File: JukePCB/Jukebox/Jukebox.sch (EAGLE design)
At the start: 33 parts, among them J1 RJ45

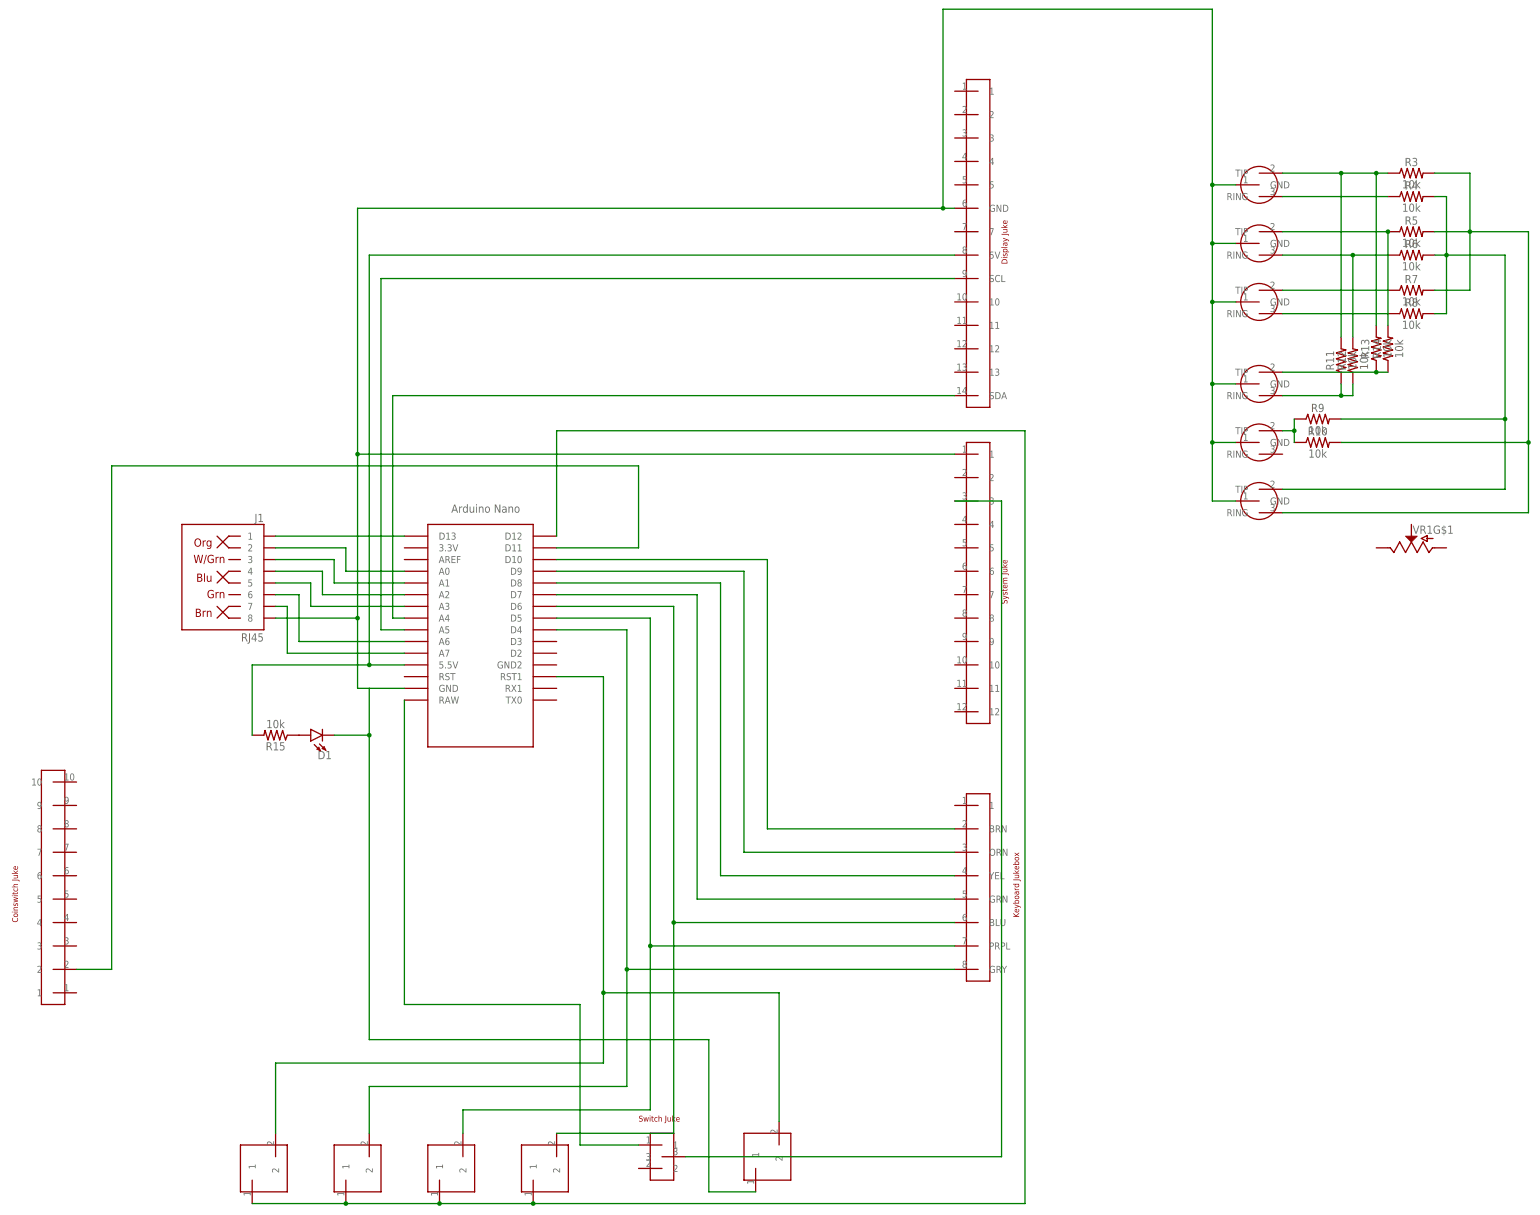
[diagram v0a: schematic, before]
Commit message: PCB UPDATE 2
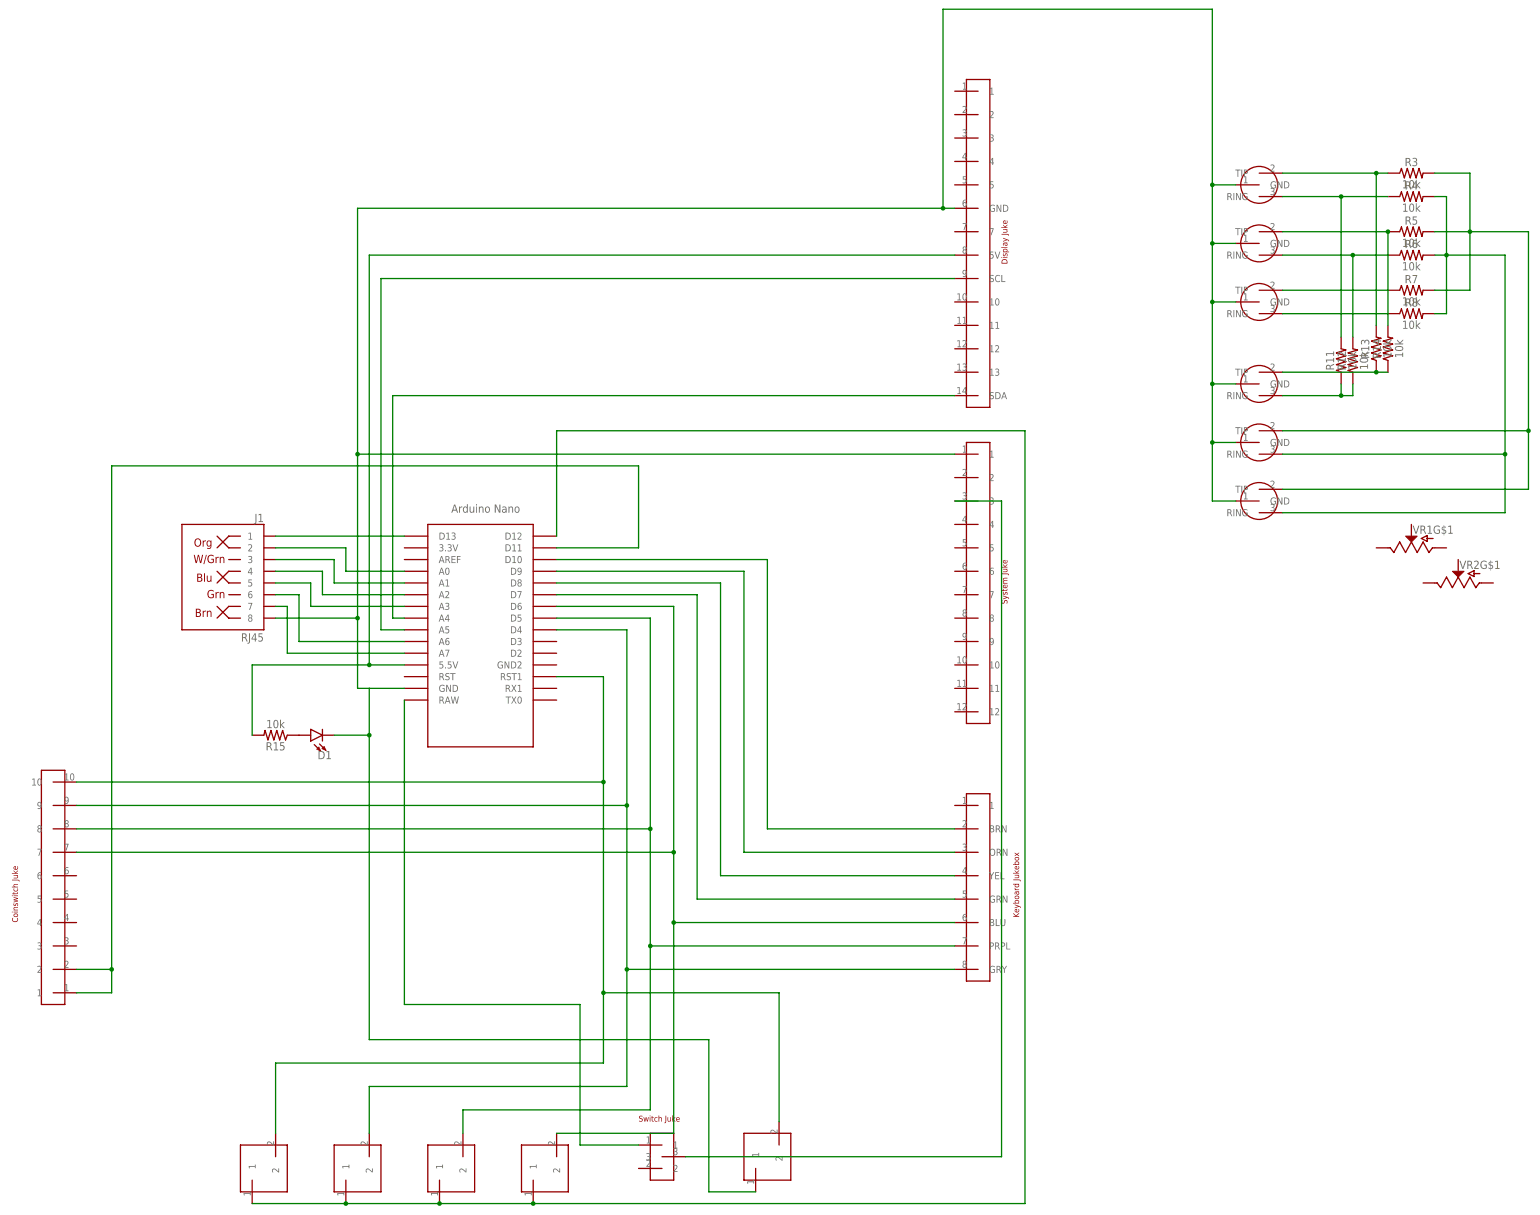
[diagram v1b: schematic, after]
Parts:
- removed R10, R9: 10k, SparkFun-Resistors:10KOHM-HORIZ-1/4W-1%
- added VR2: (no value), SparkFun-Resistors:POTENTIOMETER_DUAL-PTH-12MM-1/20W-20%
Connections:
- removed net N$22: R10.1, R9.1, U$16.TIP
- net N$1: now also U$5.9
- net N$11: now also U$5.1
- net N$14: no longer R11.2
- net N$15: now also R11.2
- net N$2: now also U$5.8
- net N$23: now also U$16.RING, U$2.RING; no longer R9.2, U$2.TIP
- net N$24: now also U$16.TIP, U$2.TIP; no longer R10.2, U$2.RING
- net N$3: now also U$5.7
- net N$9: now also U$5.10
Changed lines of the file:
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@@
 <part name="R8" library="SparkFun-Resistors" deviceset="10KOHM" device="-HORIZ-1/4W-1%" value="10k"/>
 <part name="VR1" library="SparkFun-Resistors" deviceset="POTENTIOMETER_DUAL" device="-PTH-12MM-1/20W-20%"/>
-<part name="R9" library="SparkFun-Resistors" deviceset="10KOHM" device="-HORIZ-1/4W-1%" value="10k"/>
-<part name="R10" library="SparkFun-Resistors" deviceset="10KOHM" device="-HORIZ-1/4W-1%" value="10k"/>
 <part name="U$2" library="Jukebox" deviceset="JUKEHEADPHONE" device=""/>
 <part name="R11" library="SparkFun-Resistors" deviceset="10KOHM" device="-HORIZ-1/4W-1%" value="10k"/>
@@
 <part name="R15" library="SparkFun-Resistors" deviceset="10KOHM" device="-HORIZ-1/4W-1%" value="10k"/>
 <part name="D1" library="SparkFun-LED" deviceset="LED" device="5MM"/>
+<part name="VR2" library="SparkFun-Resistors" deviceset="POTENTIOMETER_DUAL" device="-PTH-12MM-1/20W-20%"/>
 </parts>
 <sheets>
@@
 <instance part="R8" gate="G$1" x="226.06" y="55.88"/>
 <instance part="VR1" gate="G$1" x="226.06" y="5.08" rot="R90"/>
-<instance part="R9" gate="G$1" x="205.74" y="33.02"/>
-<instance part="R10" gate="G$1" x="205.74" y="27.94"/>
 <instance part="U$2" gate="G$1" x="193.04" y="15.24" rot="R90"/>
 <instance part="R11" gate="G$1" x="210.82" y="45.72" rot="R90"/>
@@
 <instance part="R15" gate="G$1" x="-20.32" y="-35.56" rot="R180"/>
 <instance part="D1" gate="G$1" x="-12.7" y="-35.56" rot="R90"/>
+<instance part="VR2" gate="G$1" x="236.22" y="-2.54" rot="R90"/>
 </instances>
 <busses>
@@
 <pinref part="U$6" gate="G$1" pin="GRY"/>
 <wire x1="127" y1="-86.36" x2="55.88" y2="-86.36" width="0.1524" layer="91"/>
-<wire x1="55.88" y1="-86.36" x2="55.88" y2="-12.7" width="0.1524" layer="91"/>
+<wire x1="55.88" y1="-86.36" x2="55.88" y2="-50.8" width="0.1524" layer="91"/>
 <pinref part="U$1" gate="G$1" pin="D4"/>
+<wire x1="55.88" y1="-50.8" x2="55.88" y2="-12.7" width="0.1524" layer="91"/>
 <wire x1="55.88" y1="-12.7" x2="40.64" y2="-12.7" width="0.1524" layer="91"/>
 <pinref part="U$10" gate="G$1" pin="2"/>
@@
 <wire x1="55.88" y1="-111.76" x2="55.88" y2="-86.36" width="0.1524" layer="91"/>
 <junction x="55.88" y="-86.36"/>
+<pinref part="U$5" gate="G$1" pin="9"/>
+<wire x1="-63.5" y1="-50.8" x2="55.88" y2="-50.8" width="0.1524" layer="91"/>
+<junction x="55.88" y="-50.8"/>
 </segment>
 </net>
@@
 <pinref part="U$6" gate="G$1" pin="PRPL"/>
 <wire x1="127" y1="-81.28" x2="60.96" y2="-81.28" width="0.1524" layer="91"/>
-<wire x1="60.96" y1="-81.28" x2="60.96" y2="-10.16" width="0.1524" layer="91"/>
+<wire x1="60.96" y1="-81.28" x2="60.96" y2="-55.88" width="0.1524" layer="91"/>
 <pinref part="U$1" gate="G$1" pin="D5"/>
+<wire x1="60.96" y1="-55.88" x2="60.96" y2="-10.16" width="0.1524" layer="91"/>
 <wire x1="60.96" y1="-10.16" x2="40.64" y2="-10.16" width="0.1524" layer="91"/>
 <pinref part="U$11" gate="G$1" pin="2"/>
@@
 <wire x1="60.96" y1="-116.84" x2="60.96" y2="-81.28" width="0.1524" layer="91"/>
 <junction x="60.96" y="-81.28"/>
+<pinref part="U$5" gate="G$1" pin="8"/>
+<wire x1="-63.5" y1="-55.88" x2="60.96" y2="-55.88" width="0.1524" layer="91"/>
+<junction x="60.96" y="-55.88"/>
 </segment>
 </net>
@@
 <pinref part="U$6" gate="G$1" pin="BLU"/>
 <wire x1="127" y1="-76.2" x2="66.04" y2="-76.2" width="0.1524" layer="91"/>
-<wire x1="66.04" y1="-76.2" x2="66.04" y2="-7.62" width="0.1524" layer="91"/>
+<wire x1="66.04" y1="-76.2" x2="66.04" y2="-60.96" width="0.1524" layer="91"/>
 <pinref part="U$1" gate="G$1" pin="D6"/>
+<wire x1="66.04" y1="-60.96" x2="66.04" y2="-7.62" width="0.1524" layer="91"/>
 <wire x1="66.04" y1="-7.62" x2="40.64" y2="-7.62" width="0.1524" layer="91"/>
 <pinref part="U$12" gate="G$1" pin="2"/>
@@
 <wire x1="66.04" y1="-121.92" x2="66.04" y2="-76.2" width="0.1524" layer="91"/>
 <junction x="66.04" y="-76.2"/>
+<pinref part="U$5" gate="G$1" pin="7"/>
+<wire x1="-63.5" y1="-60.96" x2="66.04" y2="-60.96" width="0.1524" layer="91"/>
+<junction x="66.04" y="-60.96"/>
 </segment>
 </net>
@@
 <wire x1="88.9" y1="-119.38" x2="88.9" y2="-91.44" width="0.1524" layer="91"/>
 <wire x1="88.9" y1="-91.44" x2="50.8" y2="-91.44" width="0.1524" layer="91"/>
-<wire x1="50.8" y1="-91.44" x2="50.8" y2="-22.86" width="0.1524" layer="91"/>
+<wire x1="50.8" y1="-91.44" x2="50.8" y2="-45.72" width="0.1524" layer="91"/>
 <pinref part="U$1" gate="G$1" pin="RST1"/>
+<wire x1="50.8" y1="-45.72" x2="50.8" y2="-22.86" width="0.1524" layer="91"/>
 <wire x1="50.8" y1="-22.86" x2="40.64" y2="-22.86" width="0.1524" layer="91"/>
 <pinref part="U$9" gate="G$1" pin="2"/>
@@
 <wire x1="50.8" y1="-106.68" x2="50.8" y2="-91.44" width="0.1524" layer="91"/>
 <junction x="50.8" y="-91.44"/>
+<pinref part="U$5" gate="G$1" pin="10"/>
+<wire x1="-63.5" y1="-45.72" x2="50.8" y2="-45.72" width="0.1524" layer="91"/>
+<junction x="50.8" y="-45.72"/>
 </segment>
 </net>
@@
 <pinref part="U$5" gate="G$1" pin="2"/>
 <wire x1="-55.88" y1="-86.36" x2="-63.5" y2="-86.36" width="0.1524" layer="91"/>
+<pinref part="U$5" gate="G$1" pin="1"/>
+<wire x1="-63.5" y1="-91.44" x2="-55.88" y2="-91.44" width="0.1524" layer="91"/>
+<wire x1="-55.88" y1="-91.44" x2="-55.88" y2="-86.36" width="0.1524" layer="91"/>
+<junction x="-55.88" y="-86.36"/>
 </segment>
 </net>
@@
 <segment>
 <pinref part="AUXIN" gate="G$1" pin="TIP"/>
-<wire x1="198.12" y1="86.36" x2="210.82" y2="86.36" width="0.1524" layer="91"/>
+<wire x1="198.12" y1="86.36" x2="218.44" y2="86.36" width="0.1524" layer="91"/>
 <pinref part="R3" gate="G$1" pin="1"/>
-<wire x1="210.82" y1="86.36" x2="218.44" y2="86.36" width="0.1524" layer="91"/>
 <wire x1="218.44" y1="86.36" x2="220.98" y2="86.36" width="0.1524" layer="91"/>
 <wire x1="218.44" y1="86.36" x2="218.44" y2="53.34" width="0.1524" layer="91"/>
 <junction x="218.44" y="86.36"/>
 <pinref part="R13" gate="G$1" pin="2"/>
+</segment>
+</net>
+<net name="N$15" class="0">
+<segment>
+<pinref part="AUXIN" gate="G$1" pin="RING"/>
+<wire x1="198.12" y1="81.28" x2="210.82" y2="81.28" width="0.1524" layer="91"/>
+<pinref part="R4" gate="G$1" pin="1"/>
 <pinref part="R11" gate="G$1" pin="2"/>
-<wire x1="210.82" y1="50.8" x2="210.82" y2="86.36" width="0.1524" layer="91"/>
-<junction x="210.82" y="86.36"/>
-</segment>
-</net>
-<net name="N$15" class="0">
-<segment>
-<pinref part="AUXIN" gate="G$1" pin="RING"/>
-<wire x1="198.12" y1="81.28" x2="220.98" y2="81.28" width="0.1524" layer="91"/>
-<pinref part="R4" gate="G$1" pin="1"/>
+<wire x1="210.82" y1="81.28" x2="220.98" y2="81.28" width="0.1524" layer="91"/>
+<wire x1="210.82" y1="50.8" x2="210.82" y2="81.28" width="0.1524" layer="91"/>
+<junction x="210.82" y="81.28"/>
 </segment>
 </net>
@@
 </segment>
 </net>
-<net name="N$22" class="0">
-<segment>
-<pinref part="U$16" gate="G$1" pin="TIP"/>
-<wire x1="198.12" y1="30.48" x2="200.66" y2="30.48" width="0.1524" layer="91"/>
-<pinref part="R9" gate="G$1" pin="1"/>
-<wire x1="200.66" y1="30.48" x2="200.66" y2="33.02" width="0.1524" layer="91"/>
-<pinref part="R10" gate="G$1" pin="1"/>
-<wire x1="200.66" y1="30.48" x2="200.66" y2="27.94" width="0.1524" layer="91"/>
-<junction x="200.66" y="30.48"/>
-</segment>
-</net>
 <net name="N$23" class="0">
 <segment>
-<pinref part="R9" gate="G$1" pin="2"/>
 <pinref part="R8" gate="G$1" pin="2"/>
 <wire x1="231.14" y1="55.88" x2="233.68" y2="55.88" width="0.1524" layer="91"/>
@@
 <wire x1="233.68" y1="81.28" x2="231.14" y2="81.28" width="0.1524" layer="91"/>
 <wire x1="233.68" y1="68.58" x2="246.38" y2="68.58" width="0.1524" layer="91"/>
-<wire x1="246.38" y1="68.58" x2="246.38" y2="33.02" width="0.1524" layer="91"/>
-<pinref part="U$2" gate="G$1" pin="TIP"/>
-<wire x1="246.38" y1="33.02" x2="246.38" y2="17.78" width="0.1524" layer="91"/>
-<wire x1="198.12" y1="17.78" x2="246.38" y2="17.78" width="0.1524" layer="91"/>
-<wire x1="210.82" y1="33.02" x2="246.38" y2="33.02" width="0.1524" layer="91"/>
-<junction x="246.38" y="33.02"/>
+<wire x1="246.38" y1="68.58" x2="246.38" y2="25.4" width="0.1524" layer="91"/>
+<pinref part="U$16" gate="G$1" pin="RING"/>
+<wire x1="198.12" y1="25.4" x2="246.38" y2="25.4" width="0.1524" layer="91"/>
+<pinref part="U$2" gate="G$1" pin="RING"/>
+<wire x1="198.12" y1="12.7" x2="246.38" y2="12.7" width="0.1524" layer="91"/>
+<wire x1="246.38" y1="12.7" x2="246.38" y2="25.4" width="0.1524" layer="91"/>
+<junction x="246.38" y="25.4"/>
 </segment>
 </net>
 <net name="N$24" class="0">
 <segment>
-<pinref part="R10" gate="G$1" pin="2"/>
 <pinref part="R3" gate="G$1" pin="2"/>
 <wire x1="231.14" y1="86.36" x2="238.76" y2="86.36" width="0.1524" layer="91"/>
@@
 <pinref part="R7" gate="G$1" pin="2"/>
 <wire x1="238.76" y1="60.96" x2="231.14" y2="60.96" width="0.1524" layer="91"/>
-<pinref part="U$2" gate="G$1" pin="RING"/>
-<wire x1="198.12" y1="12.7" x2="251.46" y2="12.7" width="0.1524" layer="91"/>
-<wire x1="251.46" y1="12.7" x2="251.46" y2="27.94" width="0.1524" layer="91"/>
-<wire x1="251.46" y1="27.94" x2="251.46" y2="73.66" width="0.1524" layer="91"/>
+<wire x1="251.46" y1="30.48" x2="251.46" y2="73.66" width="0.1524" layer="91"/>
 <wire x1="251.46" y1="73.66" x2="238.76" y2="73.66" width="0.1524" layer="91"/>
-<wire x1="210.82" y1="27.94" x2="251.46" y2="27.94" width="0.1524" layer="91"/>
-<junction x="251.46" y="27.94"/>
-</segment>
-</net>
+<pinref part="U$16" gate="G$1" pin="TIP"/>
+<wire x1="198.12" y1="30.48" x2="251.46" y2="30.48" width="0.1524" layer="91"/>
+<pinref part="U$2" gate="G$1" pin="TIP"/>
+<wire x1="198.12" y1="17.78" x2="251.46" y2="17.78" width="0.1524" layer="91"/>
+<wire x1="251.46" y1="17.78" x2="251.46" y2="30.48" width="0.1524" layer="91"/>
+<junction x="251.46" y="30.48"/>
+</segment>
+</net>
